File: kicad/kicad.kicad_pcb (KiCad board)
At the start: 2 copper layers, 100 x 100 mm, 108 parts, among them J101 DEBUG_LED_CONN, J102 EPD_SPI_CONN, J103 HPC_CONN, J104 STORAGE_CONN, J105 USBC_CONN, J106 GLOBAL_CONN, J107 INPUT_CONN, J108 CHARGER_CONN, J201 USB_C_Receptacle_USB2.0_16P, J301 BATTERY_CONN, J501 MOTOR_P_SF, J502 MOTOR_N_SF, Q301 2N7002, Q401 SI1308EDL, SW701 PLACEHOLDER_BT1, SW702 PLACEHOLDER_BT2, SW703 PLACEHOLDER_BT3, SW704 BT1, SW705 BT2, SW706 BT3, SW707 BT4, U201 TPD2S300, U301 BQ21061, U501 DA7280, U601 M95P32

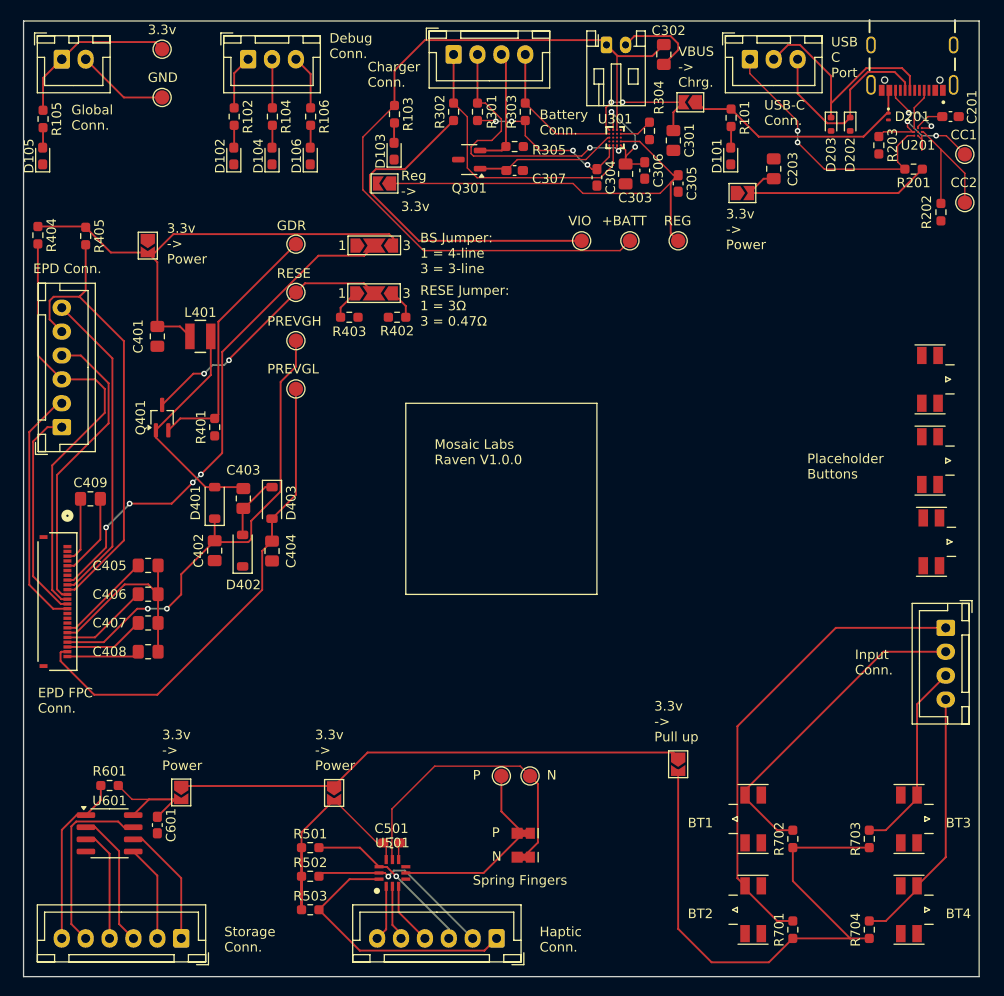
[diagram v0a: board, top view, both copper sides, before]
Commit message: silkscreen art!
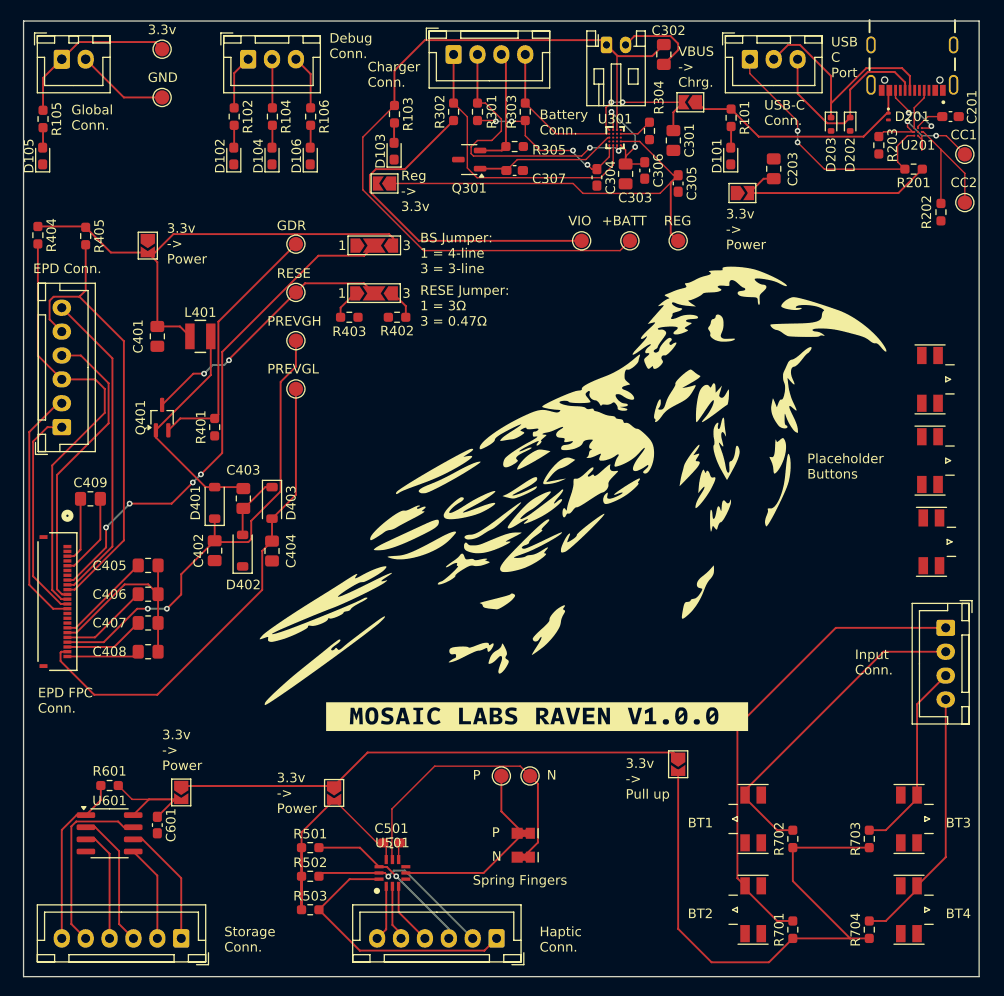
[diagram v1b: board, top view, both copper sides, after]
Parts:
- added G***: LOGO, LOGO, F.Cu at (150.4, 106.6)
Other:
- board text removed: "Mosaic Labs Raven V1.0.0"
